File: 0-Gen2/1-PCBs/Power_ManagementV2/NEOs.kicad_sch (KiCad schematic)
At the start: 36 parts

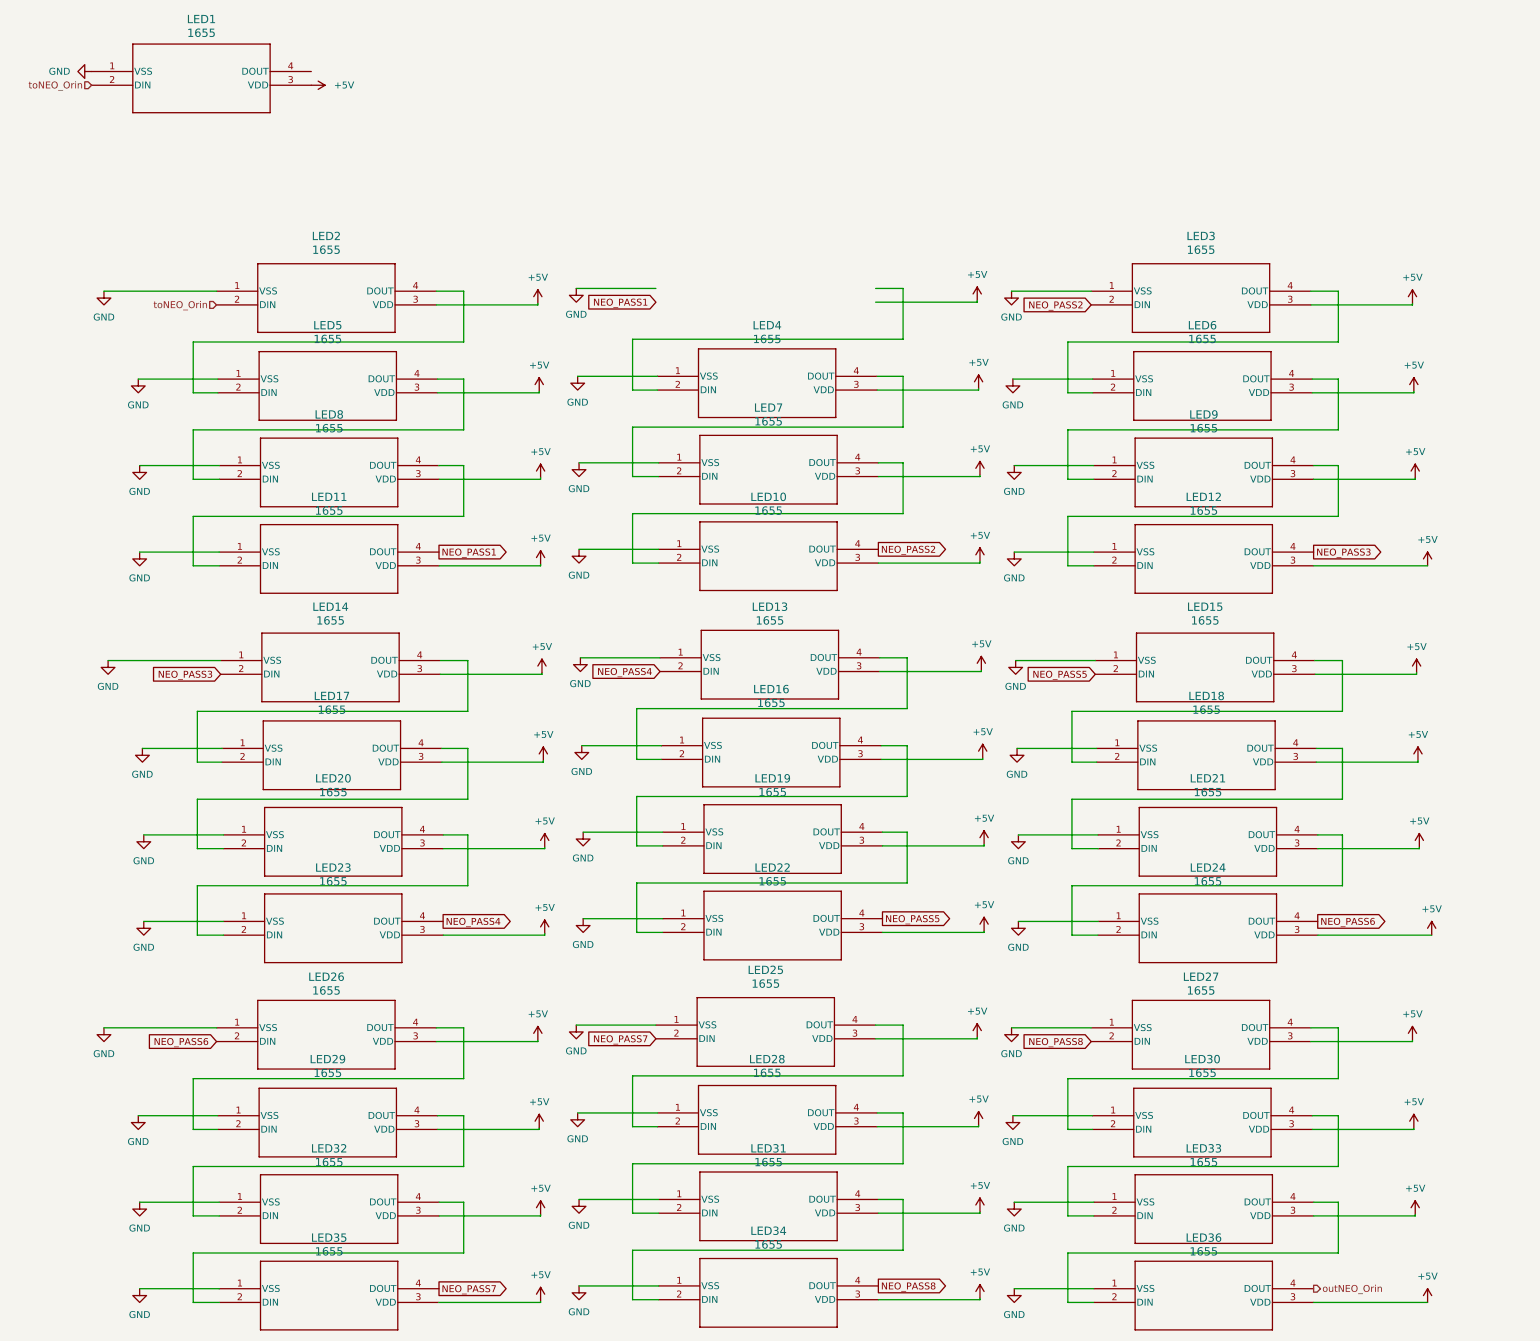
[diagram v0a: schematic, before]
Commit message: done with dist
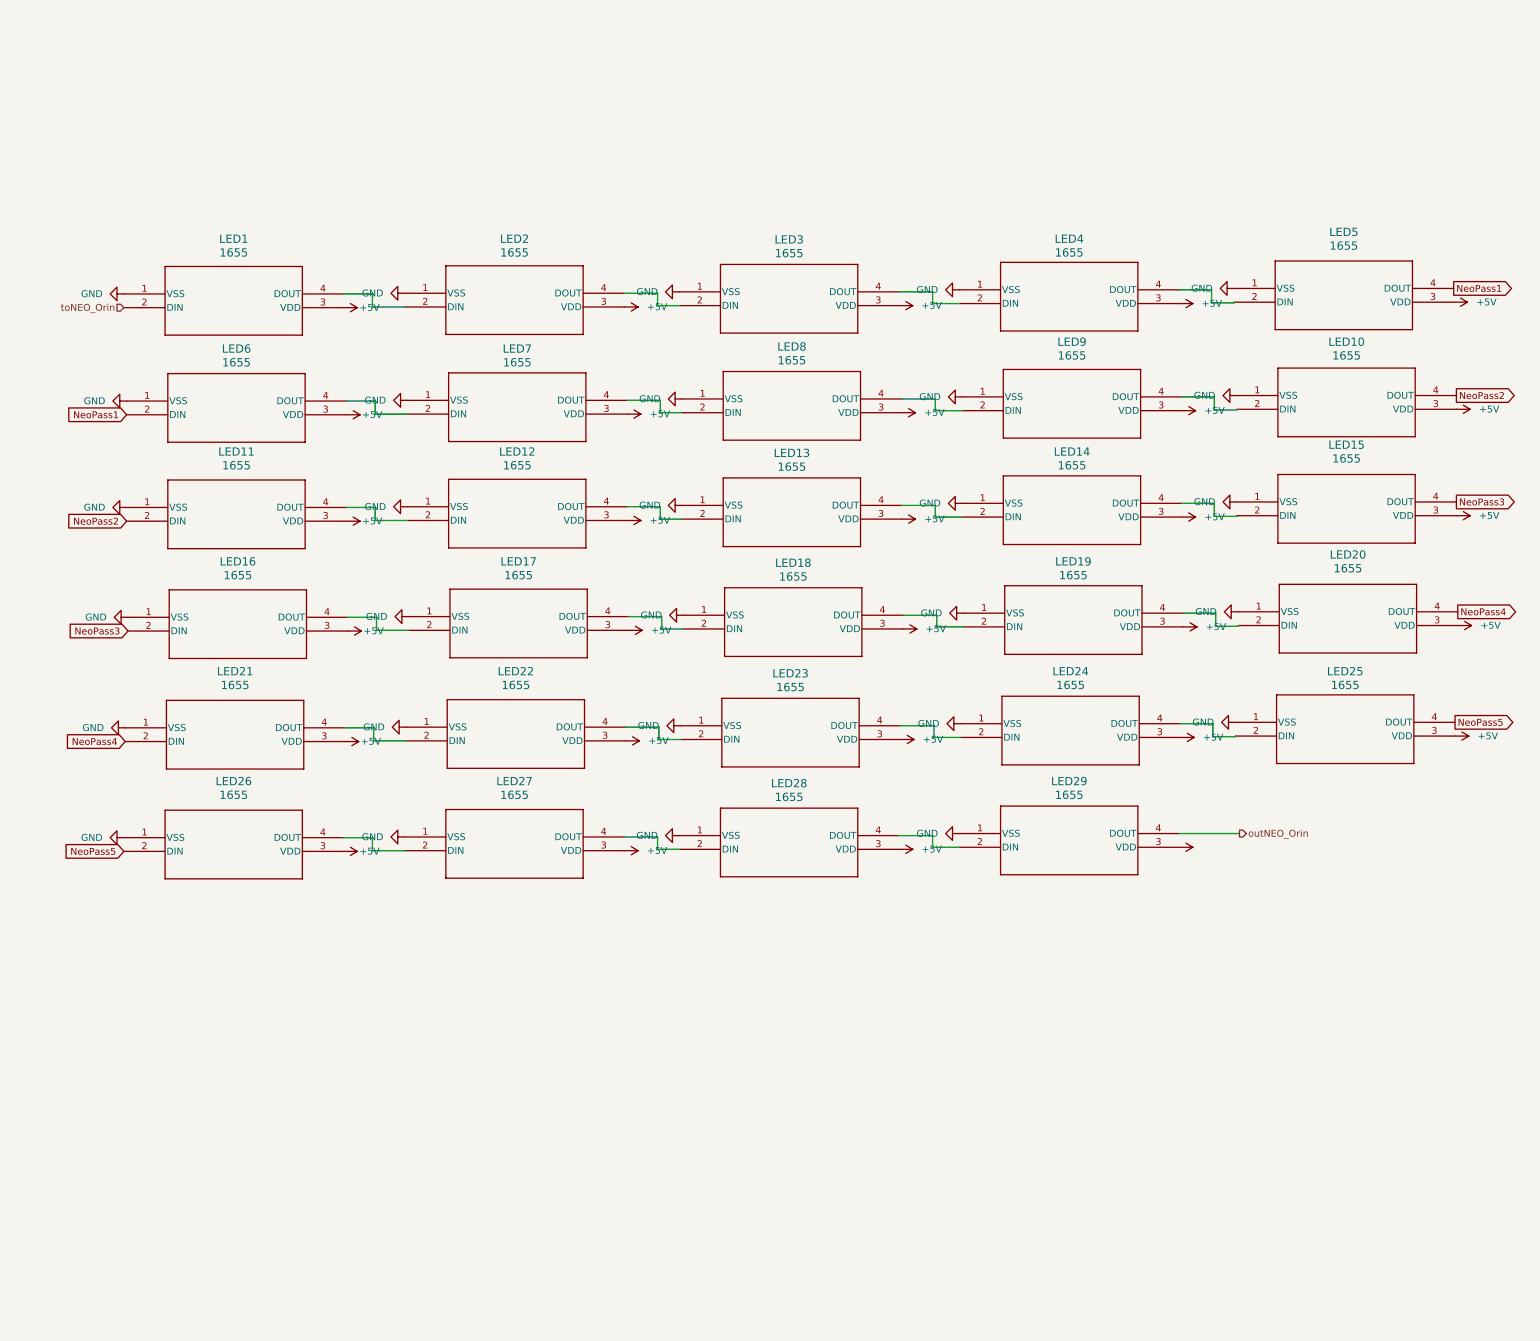
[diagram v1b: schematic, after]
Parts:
- removed LED30, LED31, LED32, LED33, LED34, LED35, LED36: 1655, LED_SMD:LED_LiteOn_LTST-E563C_PLCC4_5.0x5.0mm_P3.2mm_HandSoldering, symbol Imported_Symbols:1655
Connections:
- net NEO_PASS1 is gone; now on an unnamed net: LED11.4 (DOUT)
- net NEO_PASS7 is gone; now on an unnamed net: LED25.2 (DIN)
- net outNEO_Orin: now also LED29.4 (DOUT)
- net toNEO_Orin: no longer LED2.2 (DIN)
- net at LED22.2 (DIN): now also LED21.4 (DOUT); no longer LED19.4 (DOUT)
- net at LED3.4 (DOUT): now also LED4.2 (DIN); no longer LED6.2 (DIN)
- net at LED12.2 (DIN): no longer LED9.4 (DOUT)
- net at LED29.2 (DIN): now also LED28.4 (DOUT); no longer LED26.4 (DOUT)
- net at LED18.2 (DIN): now also LED17.4 (DOUT); no longer LED15.4 (DOUT)
- net at LED7.2 (DIN): now also LED6.4 (DOUT); no longer LED4.4 (DOUT)
- net at LED27.4 (DOUT): now also LED28.2 (DIN)
- net at LED18.4 (DOUT): now also LED19.2 (DIN); no longer LED21.2 (DIN)
- net at LED24.2 (DIN): now also LED23.4 (DOUT); no longer LED21.4 (DOUT)
- net at LED1.4 (DOUT): now also LED2.2 (DIN)
- net at LED13.4 (DOUT): now also LED14.2 (DIN); no longer LED16.2 (DIN)
- net at LED16.4 (DOUT): now also LED17.2 (DIN); no longer LED19.2 (DIN)
- net at LED8.2 (DIN): now also LED7.4 (DOUT); no longer LED5.4 (DOUT)
- net at LED8.4 (DOUT): now also LED9.2 (DIN); no longer LED11.2 (DIN)
- net at LED10.2 (DIN): now also LED9.4 (DOUT); no longer LED7.4 (DOUT)
- net at LED5.2 (DIN): now also LED4.4 (DOUT); no longer LED2.4 (DOUT)
- net at LED14.4 (DOUT): now also LED15.2 (DIN); no longer LED17.2 (DIN)
- net at LED20.2 (DIN): now also LED19.4 (DOUT); no longer LED17.4 (DOUT)
- net at LED23.2 (DIN): now also LED22.4 (DOUT); no longer LED20.4 (DOUT)
- net NeoPass5: now reaches LED25.4 (DOUT)
- net NeoPass5: now also LED26.2 (DIN); no longer LED28.2 (DIN)
- net NEO_PASS2: no longer names the net of LED3.2 (DIN)
- net NEO_PASS2: now also LED2.4 (DOUT); no longer LED10.4 (DOUT)
- net NEO_PASS3: no longer names the net of LED12.4 (DOUT)
- net NEO_PASS3: now also LED13.2 (DIN); no longer LED14.2 (DIN)
- removed net NEO_PASS4: LED13.2 (DIN), LED23.4 (DOUT)
- removed net NEO_PASS5: LED15.2 (DIN), LED22.4 (DOUT)
- net NEO_PASS6: no longer names the net of LED24.4 (DOUT)
- net NEO_PASS6: no longer LED26.2 (DIN)
- net NEO_PASS8: no longer names the net of LED27.2 (DIN)
- net NEO_PASS8: now also LED26.4 (DOUT)
- new net NeoPass1: LED5.4 (DOUT), LED6.2 (DIN)
- new net NeoPass2: LED10.4 (DOUT), LED11.2 (DIN)
- new net NeoPass3: LED15.4 (DOUT), LED16.2 (DIN)
- new net NeoPass4: LED20.4 (DOUT), LED21.2 (DIN)
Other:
- moved on the sheet: LED1
